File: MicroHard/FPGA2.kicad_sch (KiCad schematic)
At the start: 8 parts, among them U5 XC7A100T-FTG256

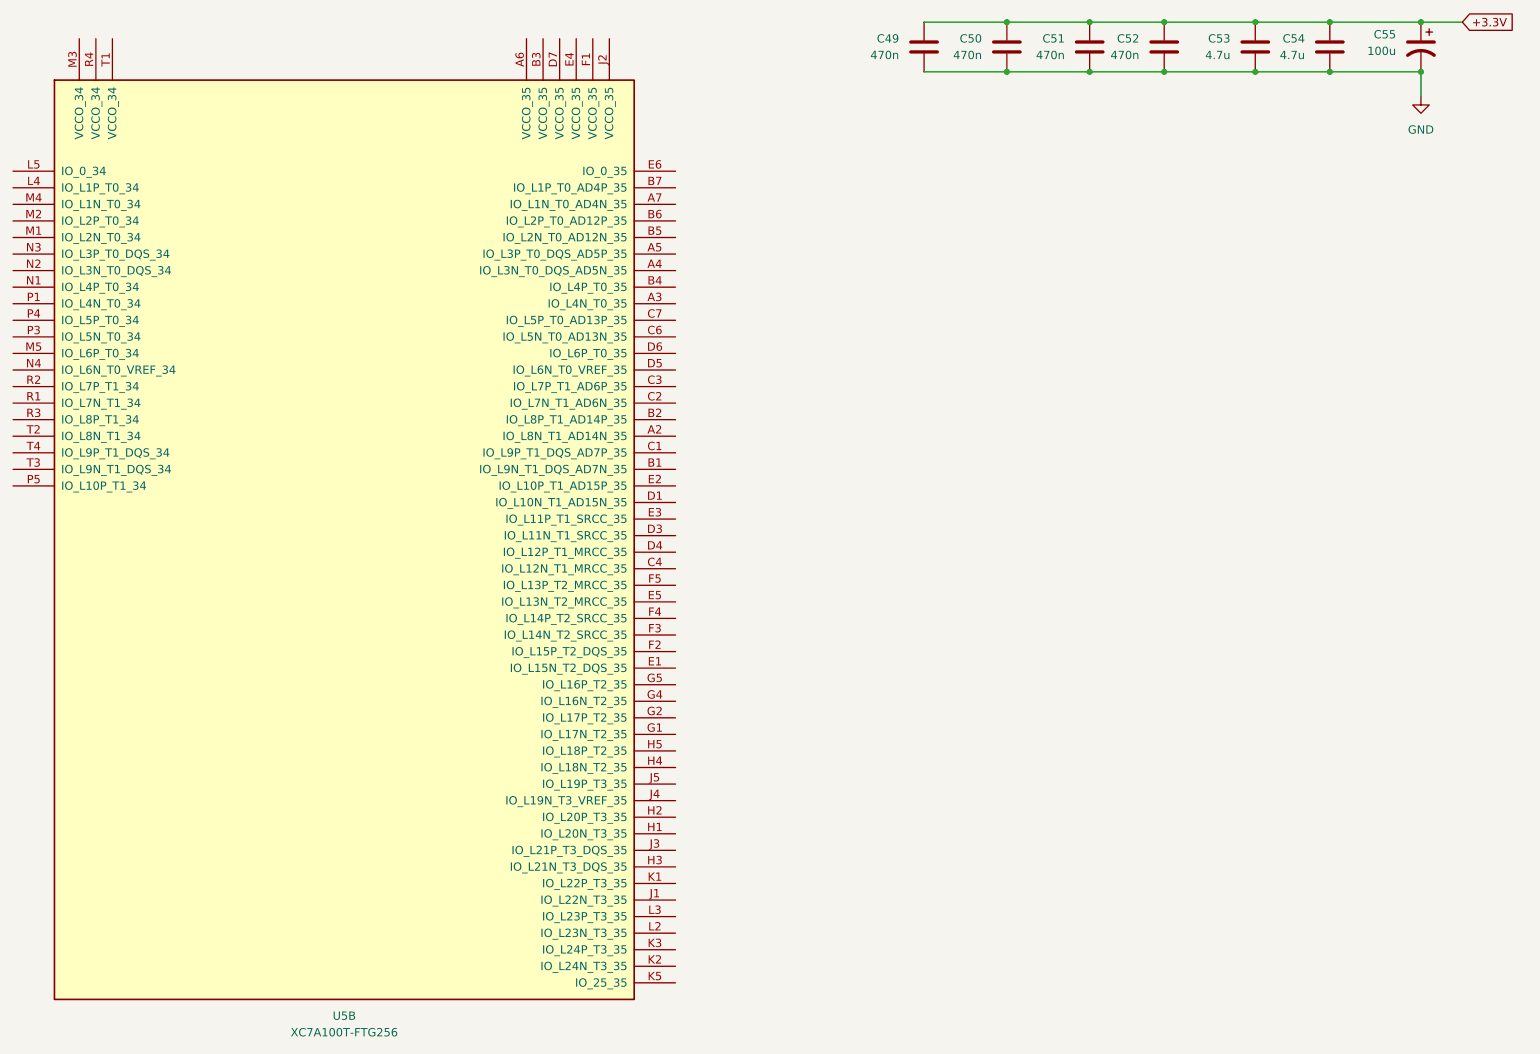
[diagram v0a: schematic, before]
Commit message: feat: finished schematic, TODO: go through checklist
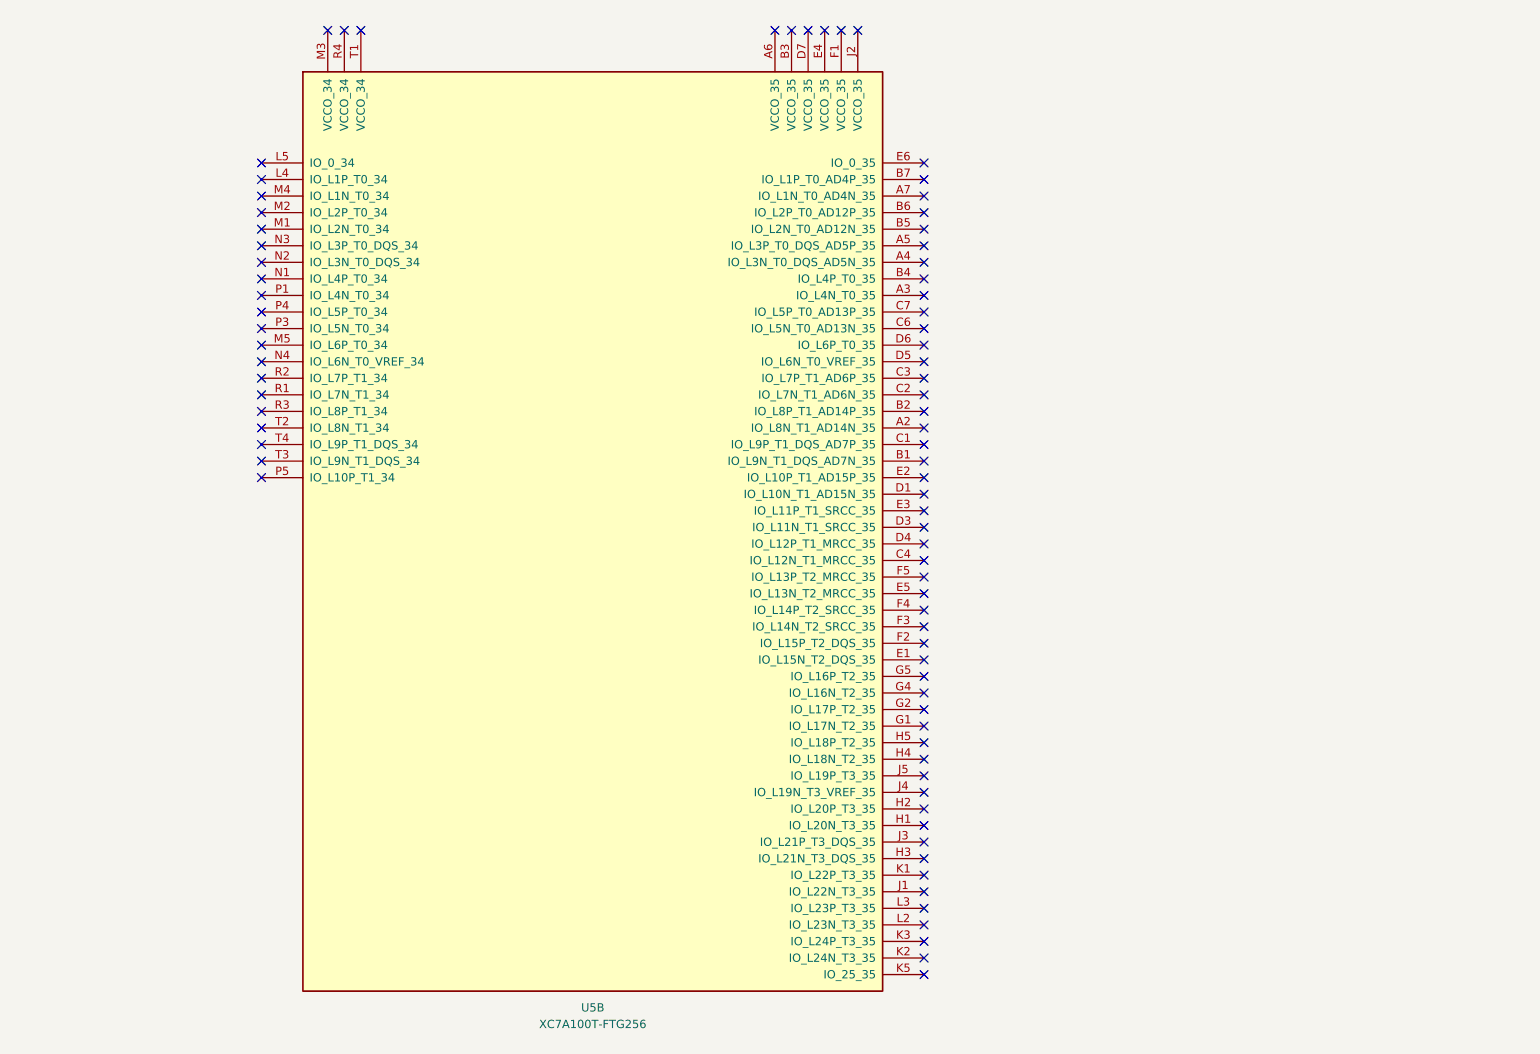
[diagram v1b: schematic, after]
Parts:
- removed C49, C50, C51, C52: 470n, symbol Device:C
- removed C53, C54: 4.7u, symbol Device:C
- removed C55: 100u, symbol Device:C_Polarized_US
- U5: footprint (none) -> MicroHard:BGA256C100P16X16_1700X1700X155
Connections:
- no-connect marks 0 -> 79
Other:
- moved on the sheet: U5B
